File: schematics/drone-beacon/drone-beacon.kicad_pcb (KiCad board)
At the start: 2 copper layers, 22.4 x 30 mm, 14 parts, among them J1 ESP32 Flashing connector, J2 Power Input, SW1 Model selection, U1 ESP32-WROOM-32U, U2 AMS1117-3.3, U3 L96

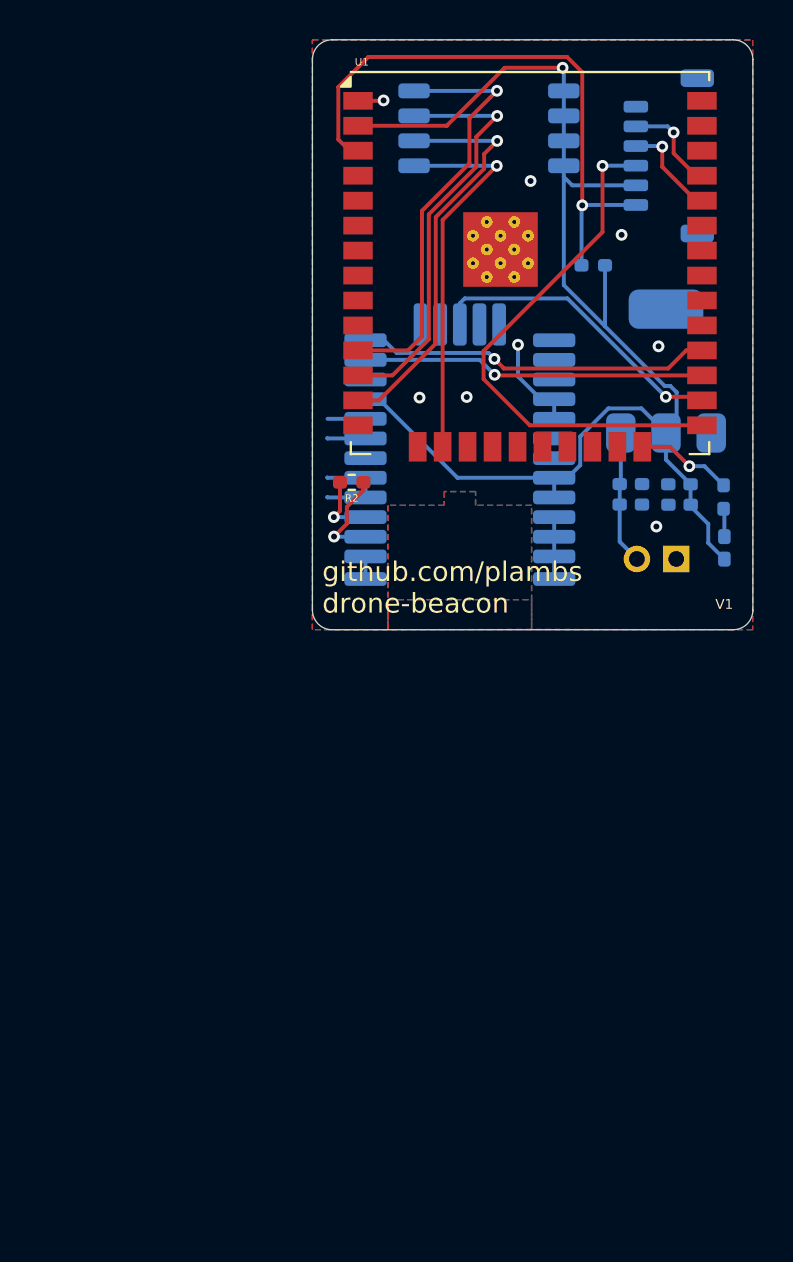
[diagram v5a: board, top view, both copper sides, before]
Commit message: Update schematics
Signed-off-by: LAMBS Pierre-Antoine <pierreantoine.lambs@gmail.com>
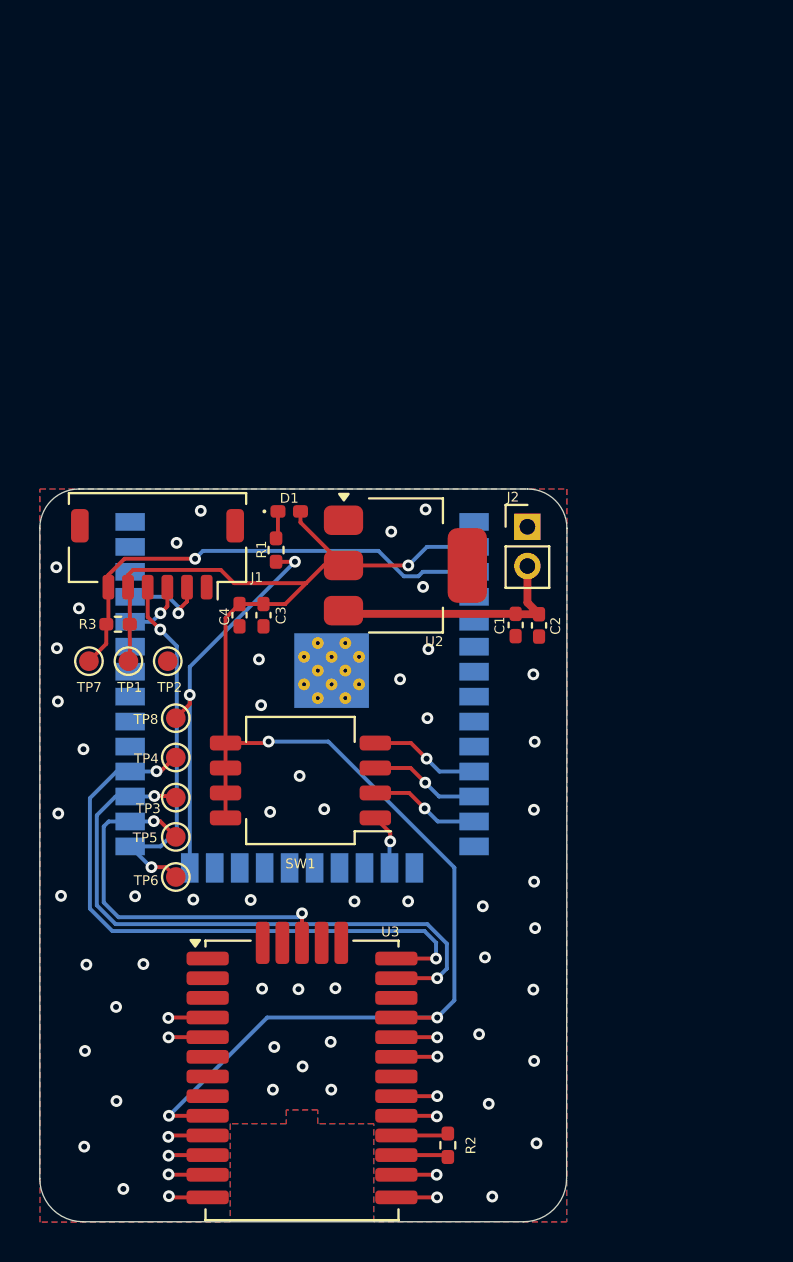
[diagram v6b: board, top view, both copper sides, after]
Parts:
- added TP1: TestPoint, TestPoint:TestPoint_Pad_D1.0mm, F.Cu at (89.7, 77.6)
- added TP2: TestPoint, TestPoint:TestPoint_Pad_D1.0mm, F.Cu at (91.7, 77.6)
- added TP3: TestPoint, TestPoint:TestPoint_Pad_D1.0mm, F.Cu at (92.2, 84.5)
- added TP4: TestPoint, TestPoint:TestPoint_Pad_D1.0mm, F.Cu at (92.2, 82.5)
- added TP5: TestPoint, TestPoint:TestPoint_Pad_D1.0mm, F.Cu at (92.2, 86.5)
- added TP6: TestPoint, TestPoint:TestPoint_Pad_D1.0mm, F.Cu at (92.2, 88.6)
- added TP7: TestPoint, TestPoint:TestPoint_Pad_D1.0mm, F.Cu at (87.7, 77.6)
- added TP8: TestPoint, TestPoint:TestPoint_Pad_D1.0mm, F.Cu at (92.2, 80.5)
- C1, C2, C3, C4, D1, J1, J2, R1, R3, SW1, U2, U3: moved to F.Cu
- U1: moved to B.Cu
- moved SW1 34.5 mm to (98.5, 83.7), turned to 180 degrees
- moved R2 34.1 mm to (106.0, 102.2), turned to -90 degrees
- moved J1 33.0 mm to (91.2, 72.2), turned to 180 degrees
- moved U3 32.5 mm to (98.6, 98.9), turned to 0 degrees
- moved R3 30.3 mm to (89.2, 75.7)
- moved U1 24.4 mm to (98.6, 78.8), turned to 180 degrees
- moved C4 23.4 mm to (95.4, 75.3), turned to -90 degrees
- moved R1 22.9 mm to (97.2, 71.9), turned to 90 degrees
- moved D1 22.2 mm to (97.9, 70.0), turned to 0 degrees
- moved C3 21.9 mm to (96.6, 75.3), turned to -90 degrees
- moved U2 16.5 mm to (103.8, 72.7), turned to 0 degrees
- moved C1 9.26 mm to (109.4, 75.8), turned to -90 degrees
- moved J2 7.75 mm to (110.0, 70.8), turned to 0 degrees
- moved C2 7.72 mm to (110.6, 75.8), turned to -90 degrees
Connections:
- U3 pad 8: +3.3V -> unconnected-(U3-V_BCKP-Pad8)
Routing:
- net /DIP1: track 19.6 -> 2.88 mm
- net /DIP4: track 21.8 -> 5.63 mm
- net /DIP3: track 21.4 -> 5.63 mm
- net /DIP2: track 21.0 -> 5.63 mm
- net +3.3V: track 68.4 -> 83.7 mm, vias 1 -> 4
- net /STATUS_LED: track 4.96 -> 20.2 mm, vias 1 -> 2
- net /GPS_TX: track 17.4 -> 31.5 mm, vias 1 -> 2
- net /GPS_RX: track 18.2 -> 32.0 mm, vias 1 -> 2
- net /ESP32_BOOT: track 27.1 -> 18.7 mm, vias 1 -> 2
- net /ESP32_EN: track 30.2 -> 24.4 mm
- net /VIN: track 6.80 -> 12.5 mm
- net /GPS_PPS: track 15.6 -> 20.0 mm, vias 1 -> 2
- net GND: track 20.3 -> 24.5 mm, vias 8 -> 65
- net /RF_OUT: track 4.99 -> 2.52 mm, vias 1 -> 0
- net /ESP32_RX: track 5.12 -> 3.20 mm
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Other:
- board size 22.4 x 30 mm -> 26.8 x 37.3 mm
- board text removed: "V1"
- board text removed: "github.com/plambs drone-beacon"
